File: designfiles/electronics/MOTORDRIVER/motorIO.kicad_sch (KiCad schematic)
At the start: 3 parts, among them J2 1-84952-1, J5 1-84952-1, J7 1-84952-1

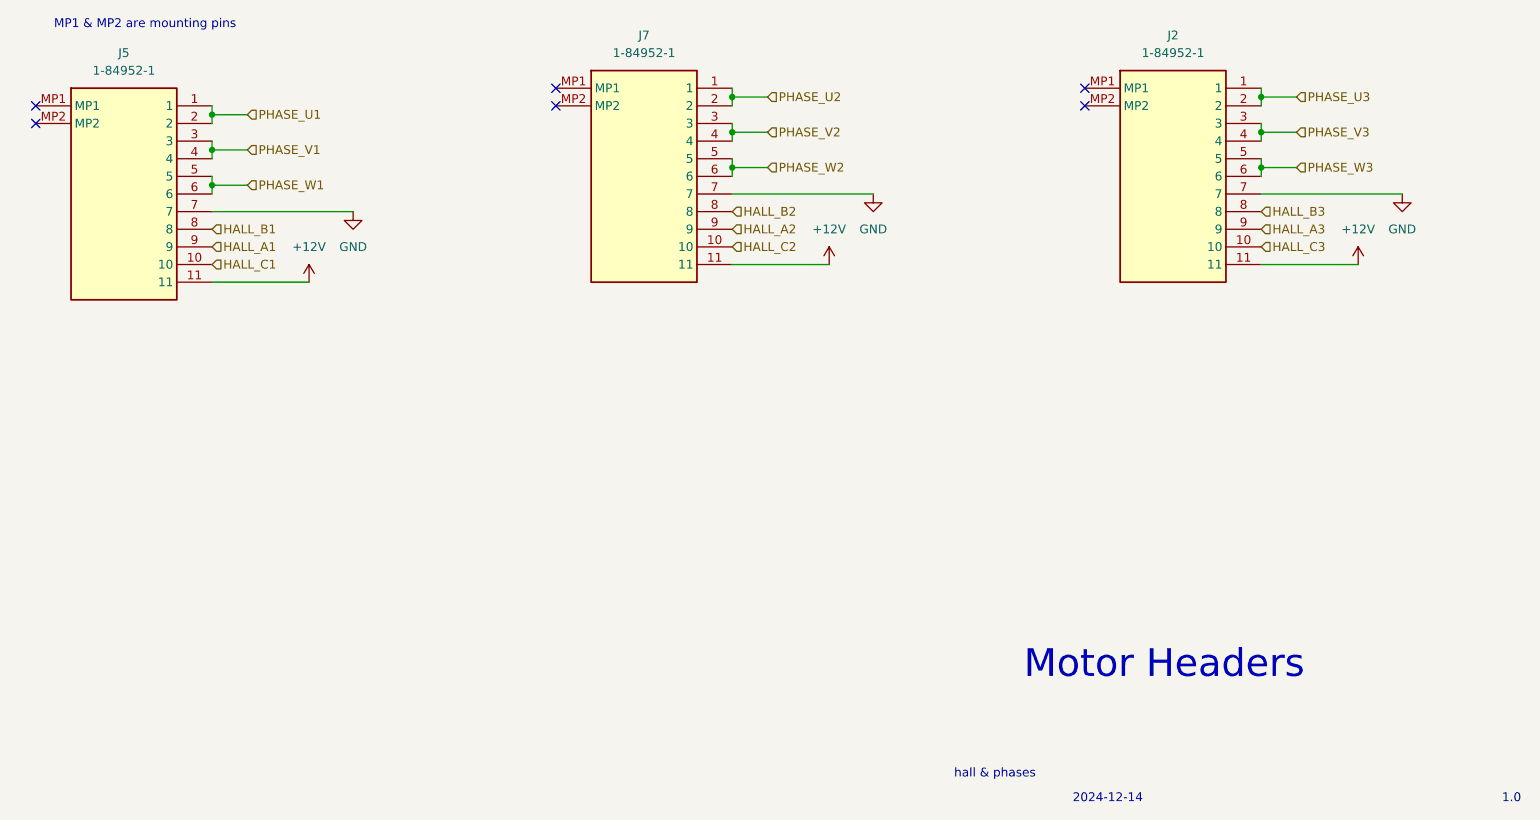
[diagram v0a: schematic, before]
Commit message: worked on pcb
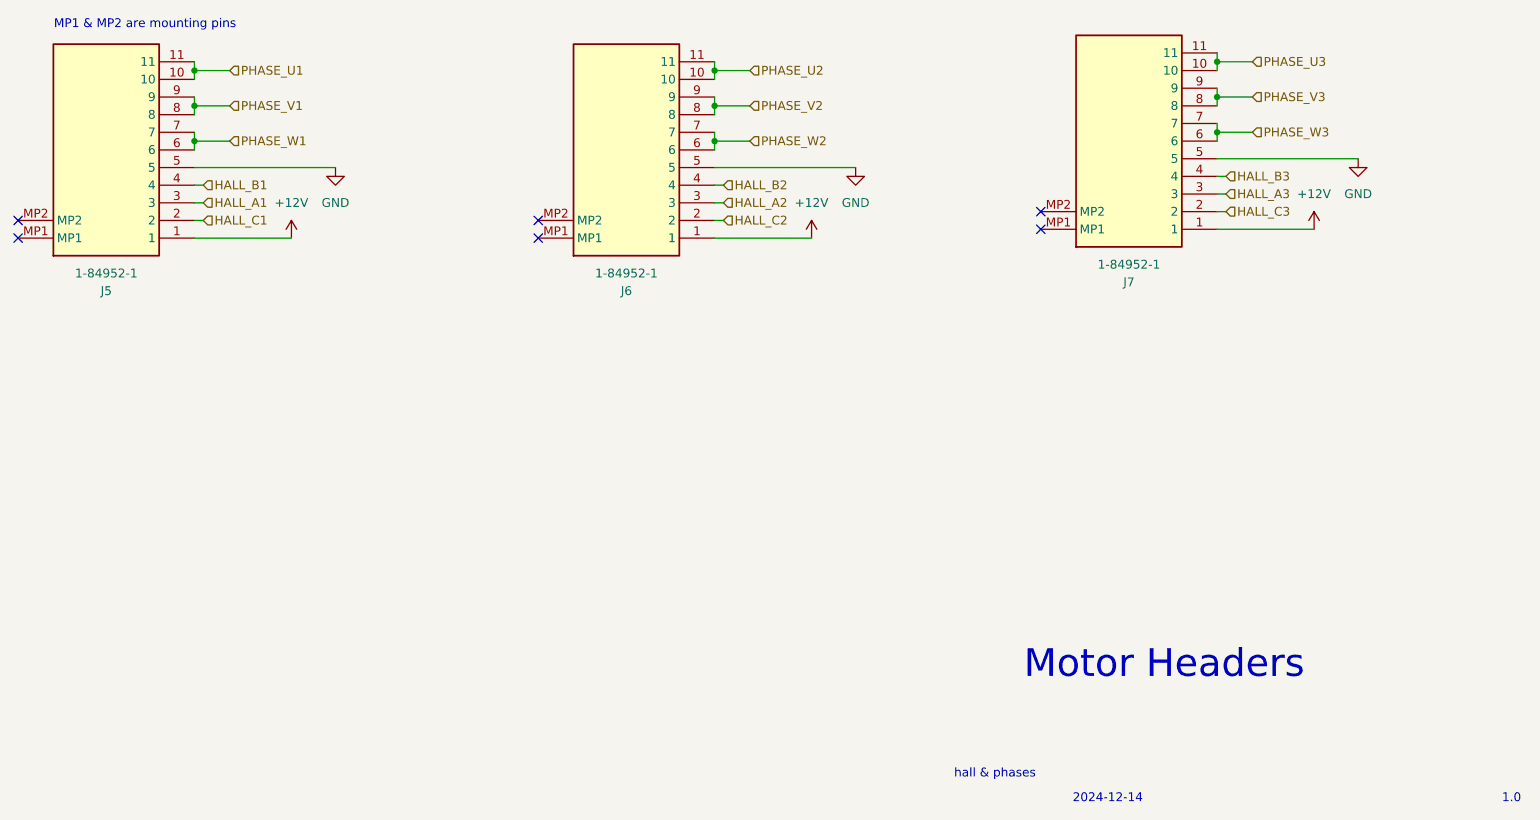
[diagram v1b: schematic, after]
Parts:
- removed J2: 1-84952-1, kuben-footprints:1849521, symbol 1-84952-1:1-84952-1
- added J7: 1-84952-1, kuben-footprints:1849521, symbol 1-84952-1:1-84952-1
- renumbered J7 to J6
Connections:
- net +12V: now also J5.1, J6.1, J7.1; no longer J5.11, J6.11
- net GND: now also J5.5, J6.5, J7.5; no longer J5.7, J6.7
- net HALL_A1: now also J5.3; no longer J5.9
- net HALL_A2: now also J6.3; no longer J6.9
- net HALL_A3: now also J7.3
- net HALL_B1: now also J5.4; no longer J5.8
- net HALL_B2: now also J6.4; no longer J6.8
- net HALL_B3: now also J7.4
- net HALL_C1: now also J5.2; no longer J5.10
- net HALL_C2: now also J6.2; no longer J6.10
- net HALL_C3: now also J7.2
- net PHASE_U1: now also J5.10, J5.11; no longer J5.1, J5.2
- net PHASE_U2: now also J6.10, J6.11; no longer J6.1, J6.2
- net PHASE_U3: now also J7.10, J7.11
- net PHASE_V1: now also J5.8, J5.9; no longer J5.3, J5.4
- net PHASE_V2: now also J6.8, J6.9; no longer J6.3, J6.4
- net PHASE_V3: now also J7.8, J7.9
- net PHASE_W1: now also J5.7; no longer J5.5
- net PHASE_W2: now also J6.7; no longer J6.5
- net PHASE_W3: now also J7.6, J7.7
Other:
- moved on the sheet: J6
